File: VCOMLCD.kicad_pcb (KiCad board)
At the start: 2 copper layers, 123.2 x 44.5 mm, 49 parts, among them J1 Screw_Terminal_01x02, J2 USB_B_Mini, J3 Conn_01x05, J4 Conn_01x03, J5 Conn_01x06, Q1 BC847, SW1 SYS_RST, SW2 BTN, U1 MCP73831-2-OT, U2 MCP1700-3302E_SOT23, U3 74LVC4245A, U4 LCD-016N002L, U5 STM32F042F4Px, U6 ESP-12E

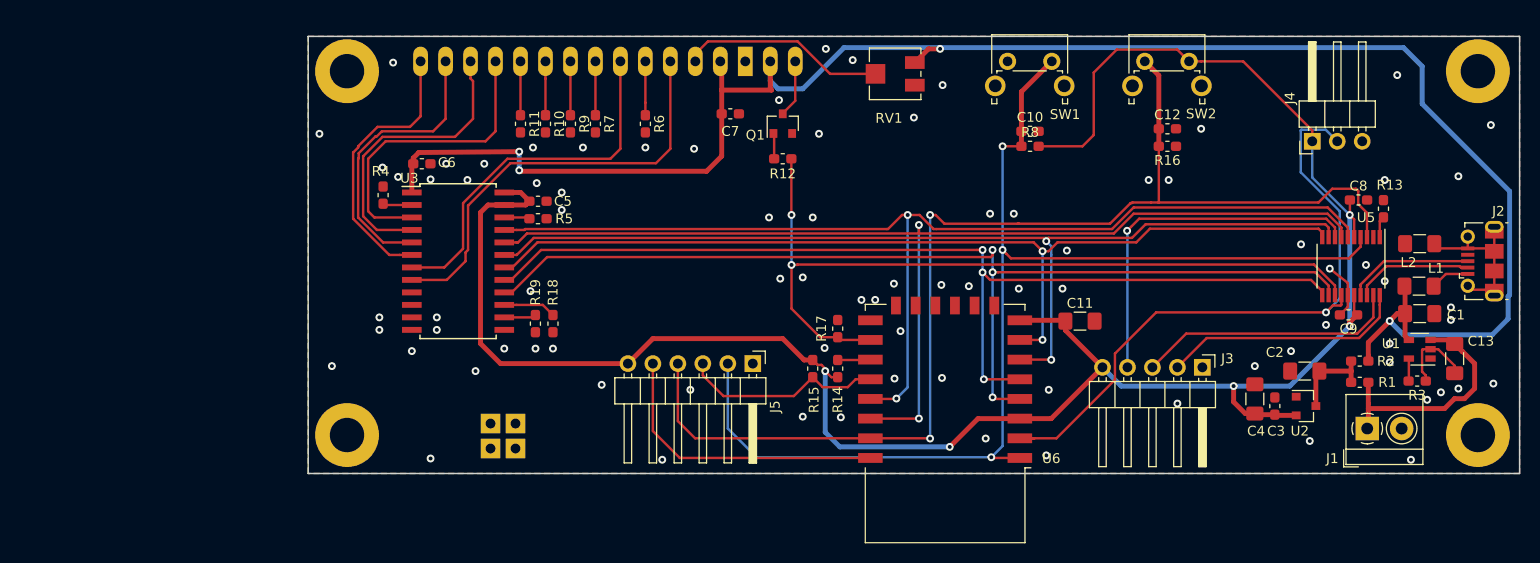
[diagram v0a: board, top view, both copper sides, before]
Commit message: pre-fabrication commit
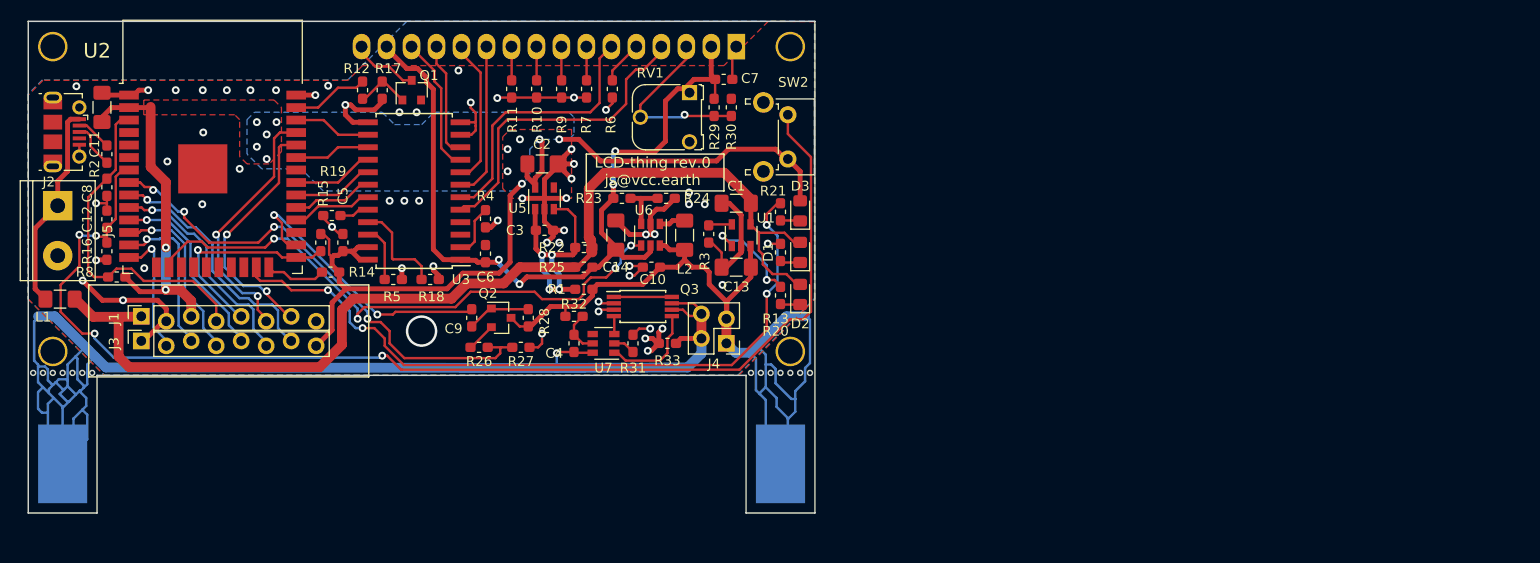
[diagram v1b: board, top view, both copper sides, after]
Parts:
- removed SW1: SYS_RST, Button_Switch_THT:SW_Tactile_SPST_Angled_PTS645Vx83-2LFS
- added C14: 10u, Capacitor_SMD:C_1206_3216Metric_Pad1.42x1.75mm_HandSolder, F.Cu at (108.8, 69.7)
- added D1: LED_RED, LED_SMD:LED_0805_2012Metric_Pad1.15x1.40mm_HandSolder, F.Cu at (127.5, 71.5)
- added D2: LED_GREEN, LED_SMD:LED_0805_2012Metric_Pad1.15x1.40mm_HandSolder, F.Cu at (127.5, 75.8)
- added D3: LED_BLUE, LED_SMD:LED_0805_2012Metric_Pad1.15x1.40mm_HandSolder, F.Cu at (127.5, 67.3)
- added Q2: AO3401A, Package_TO_SOT_SMD:SOT-23, F.Cu at (97.1, 78.2)
- added Q3: FS8205A, Package_SO:TSSOP-8_4.4x3mm_P0.65mm, F.Cu at (111.5, 77.0)
- added R20: 1k, Resistor_SMD:R_0603_1608Metric_Pad1.05x0.95mm_HandSolder, F.Cu at (125.5, 75.9)
- added R21: 200, Resistor_SMD:R_0603_1608Metric_Pad1.05x0.95mm_HandSolder, F.Cu at (125.5, 67.4)
- added R22: NC, Resistor_SMD:R_0603_1608Metric_Pad1.05x0.95mm_HandSolder, F.Cu at (105.5, 71.0)
- added R23: 698k, Resistor_SMD:R_0603_1608Metric_Pad1.05x0.95mm_HandSolder, F.Cu at (109.4, 66.0)
- added R24: 133k, Resistor_SMD:R_0603_1608Metric_Pad1.05x0.95mm_HandSolder, F.Cu at (113.9, 66.0)
- added R25: NC, Resistor_SMD:R_0603_1608Metric_Pad1.05x0.95mm_HandSolder, F.Cu at (105.5, 73.0)
- added R26: 10k/1%, Resistor_SMD:R_0603_1608Metric_Pad1.05x0.95mm_HandSolder, F.Cu at (94.8, 81.2)
- added R27: 10k/1%, Resistor_SMD:R_0603_1608Metric_Pad1.05x0.95mm_HandSolder, F.Cu at (99.1, 81.2)
- added R28: 10k, Resistor_SMD:R_0603_1608Metric_Pad1.05x0.95mm_HandSolder, F.Cu at (99.8, 78.2)
- added R29: NC, Resistor_SMD:R_0603_1608Metric_Pad1.05x0.95mm_HandSolder, F.Cu at (118.8, 56.8)
- added R30: NC, Resistor_SMD:R_0603_1608Metric_Pad1.05x0.95mm_HandSolder, F.Cu at (120.5, 56.8)
- added R31: 1k, Resistor_SMD:R_0603_1608Metric_Pad1.05x0.95mm_HandSolder, F.Cu at (110.5, 80.8)
- added R32: 200, Resistor_SMD:R_0603_1608Metric_Pad1.05x0.95mm_HandSolder, F.Cu at (104.5, 78.0)
- added R33: NC, Resistor_SMD:R_0603_1608Metric_Pad1.05x0.95mm_HandSolder, F.Cu at (114.0, 80.8)
- added TP1: Lipo+, TestPoint:TestPoint_Pad_1.0x1.0mm, B.Cu at (125.5, 93.0)
- added TP2: LiPo-, TestPoint:TestPoint_Pad_1.0x1.0mm, B.Cu at (52.5, 93.0)
- added U7: DW01x, Package_TO_SOT_SMD:SOT-23-6, F.Cu at (107.5, 80.8)
- C10, C3: value 100n -> 1u
- C11, C13, C2: value 22u -> 10u
- C4: value 22u -> 100n; footprint Capacitor_SMD:C_1206_3216Metric_Pad1.42x1.75mm_HandSolder -> Capacitor_SMD:C_0603_1608Metric_Pad1.05x0.95mm_HandSolder
- J1: value Screw_Terminal_01x02 -> Conn_01x08; footprint TerminalBlock_4Ucon:TerminalBlock_4Ucon_1x02_P3.50mm_Horizontal -> Connector_PinSocket_2.54mm:PinSocket_1x08_P2.54mm_Vertical
- J3: value Conn_01x05 -> Conn_01x08; footprint Connector_PinHeader_2.54mm:PinHeader_1x05_P2.54mm_Horizontal -> Connector_PinSocket_2.54mm:PinSocket_1x08_P2.54mm_Vertical
- J4: value Conn_01x03 -> LiPo_ext; footprint Connector_PinHeader_2.54mm:PinHeader_1x03_P2.54mm_Horizontal -> Connector_PinHeader_2.54mm:PinHeader_2x02_P2.54mm_Vertical
- J5: value Conn_01x06 -> Screw_Terminal_01x02; footprint Connector_PinHeader_2.54mm:PinHeader_1x06_P2.54mm_Horizontal -> TerminalBlock:TerminalBlock_bornier-2_P5.08mm
- L1: value L_Small -> 0R
- L2: value L_Small -> 10uH
- Q1: value BC847 -> BC817
- R1: value NC -> 0R
- R12, R16, R3, R8: value R -> 10k
- R13: value R -> 1k
- R2: value 0R -> 200
- RV1: footprint Potentiometer_SMD:Potentiometer_Vishay_TS53YJ_Vertical -> Potentiometer_THT:Potentiometer_Runtron_RM-065_Vertical
- U2: value MCP1700-3302E_SOT23 -> ESP32-WROOM-32; footprint Package_TO_SOT_SMD:SOT-23 -> RF_Module:ESP32-WROOM-32
- U4: footprint Display:LCD-016N002L -> Display:WC1602A
- U5: value STM32F042F4Px -> XC6220B331MR; footprint Package_SO:TSSOP-20_4.4x6.5mm_P0.65mm -> Package_TO_SOT_SMD:SOT-23-5
- U6: value ESP-12E -> TLV61046ADB; footprint RF_Module:ESP-12E -> Package_TO_SOT_SMD:SOT-23-6
- moved J2 144.7 mm to (52.7, 59.2), turned to 270 degrees
- moved L1 138.2 mm to (52.2, 76.2), turned to 180 degrees
- moved R2 129.1 mm to (57.0, 61.5), turned to 90 degrees
- moved C8 127.3 mm to (57.0, 64.9), turned to 270 degrees
- moved J1 125.2 mm to (60.5, 78.2), turned to 90 degrees
- moved U2 113.6 mm to (67.8, 63.8)
- moved R16 108.4 mm to (57.0, 71.4), turned to 90 degrees
- moved C12 108.2 mm to (57.0, 68.1), turned to 90 degrees
- moved J3 107.9 mm to (60.5, 80.8), turned to 90 degrees
- moved C11 101.8 mm to (56.5, 56.8), turned to 90 degrees
- moved R8 93.8 mm to (58.0, 74.0)
- moved C9 89.2 mm to (94.1, 78.2), turned to 90 degrees
- moved U5 82.3 mm to (101.5, 66.0), turned to 90 degrees
- moved C2 80.4 mm to (101.2, 62.5), turned to 0 degrees
- moved R1 79.5 mm to (105.5, 75.2)
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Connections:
- C10 pad 1: /ESP_RTS -> +BATT
- C2 pad 1: Net-(C2-Pad1) -> +3V3
- C3 pad 1: +3V3 -> Net-(C3-Pad1)
- C4 pad 1: +3V3 -> Net-(C4-Pad1)
- C4 pad 2: GND -> Net-(C4-Pad2)
- C6 pad 1: VBUS -> +5V
- C7 pad 1: VBUS -> +5V
- C8 pad 1: +3V3 -> /PROG_RTS
- C9 pad 1: +3V3 -> Net-(C9-Pad1)
- C9 pad 2: GND -> /LIPO_DIV_ENA
- J1 pad 1: +BATT -> VBUS
- J2 pad 5: Net-(J2-Pad5) -> GND
- J2 pad 6: Net-(J2-Pad5) -> GND
- J3 pad 2: /SWCLK -> /GPIO12
- J3 pad 3: /SWDIO -> /GPIO14
- J3 pad 4: /STM_TX -> /GPIO27
- J3 pad 5: +3V3 -> /GPIO26
- J4 pad 1: +3V3 -> +BATT
- J4 pad 2: Net-(J4-Pad2) -> Net-(C4-Pad2)
- J4 pad 3: GND -> +BATT
- J5 pad 1: GND -> Net-(J2-Pad1)
- J5 pad 2: /ESP_RTS -> GND
- L2 pad 1: Net-(J2-Pad5) -> +BATT
- L2 pad 2: GND -> Net-(L2-Pad2)
- R1 pad 1: Net-(C2-Pad1) -> Net-(C3-Pad1)
- R13 pad 1: GND -> Net-(D1-Pad1)
- R13 pad 2: Net-(R13-Pad2) -> GND
- R15 pad 1: /ESP_DTR -> /PROG_DTR
- R17 pad 2: /BL_CTRL -> Net-(Q1-Pad1)
- R2 pad 1: Net-(C2-Pad1) -> Net-(J2-Pad3)
- R2 pad 2: VBUS -> Net-(J2-Pad2)
- R8 pad 1: /ESP_RTS -> /PROG_RTS
- RV1 pad 1: VBUS -> +5V
- U2 pad 3: Net-(C2-Pad1) -> /PROG_RTS
- U3 pad 1: VBUS -> +5V
- U3 pad 14: Net-(R19-Pad2) -> /DB6_3V3
- U3 pad 15: Net-(R18-Pad2) -> /DB7_3V3
- U3 pad 16: Net-(U3-Pad16) -> /DB5_3V3
- U3 pad 17: Net-(U3-Pad17) -> /DB4_3V3
- U3 pad 18: Net-(U3-Pad18) -> /E_3V3
- U3 pad 19: Net-(U3-Pad19) -> /RS_3V3
- U3 pad 20: Net-(U3-Pad20) -> Net-(R19-Pad2)
- U3 pad 21: Net-(U3-Pad21) -> Net-(R18-Pad2)
- U4 pad 11: Net-(U3-Pad3) -> Net-(U3-Pad7)
- U4 pad 12: Net-(U3-Pad4) -> Net-(U3-Pad8)
- U4 pad 13: Net-(U3-Pad5) -> Net-(U3-Pad10)
- U4 pad 14: Net-(U3-Pad6) -> Net-(U3-Pad9)
- U4 pad 15: VBUS -> +5V
- U4 pad 2: VBUS -> +5V
- U4 pad 4: Net-(U3-Pad8) -> Net-(U3-Pad5)
- U4 pad 6: Net-(U3-Pad7) -> Net-(U3-Pad6)
- U5 pad 1: Net-(R13-Pad2) -> Net-(C3-Pad1)
- U5 pad 2: Net-(U5-Pad2) -> GND
- U5 pad 3: /BTN -> Net-(C3-Pad1)
- U5 pad 4: /ESP_RTS -> Net-(U5-Pad4)
- U6 pad 1: /ESP_RTS -> Net-(L2-Pad2)
- U6 pad 2: Net-(J4-Pad2) -> GND
- U6 pad 3: +3V3 -> Net-(R23-Pad2)
- U6 pad 4: Net-(U3-Pad16) -> /5V_ENA
- U6 pad 5: Net-(U3-Pad17) -> +5V
- U6 pad 6: Net-(U3-Pad19) -> +BATT
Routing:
- net Net-(C4-Pad2): track 0.00 -> 158.6 mm, vias 0 -> 1
- net /ESP_RTS: track 119.7 -> 0.00 mm, vias 3 -> 0
- net Net-(U3-Pad20): track 113.4 -> 0.00 mm, vias 2 -> 0
- net Net-(U3-Pad21): track 111.5 -> 0.00 mm, vias 2 -> 0
- net GND: track 14.0 -> 121.2 mm, vias 84 -> 57
- net Net-(U3-Pad16): track 105.3 -> 0.00 mm, vias 3 -> 0
- net Net-(U3-Pad17): track 102.5 -> 0.00 mm, vias 3 -> 0
- net Net-(U3-Pad19): track 102.2 -> 0.00 mm, vias 2 -> 0
- net +3V3: track 216.9 -> 118.9 mm, vias 5 -> 13
- net Net-(U3-Pad18): track 97.5 -> 0.00 mm, vias 2 -> 0
- net +5V: track 0.00 -> 82.3 mm, vias 0 -> 4
- net +BATT: track 24.4 -> 101.2 mm
- net VBUS: track 185.2 -> 108.7 mm, vias 4 -> 0
- net /BL_CTRL: track 81.7 -> 7.85 mm, vias 2 -> 0
- net Net-(R21-Pad1): track 0.00 -> 73.8 mm, vias 0 -> 4
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- added copper zone on B.Cu, net +3V3
- added copper zone on F.Cu, net +3V3
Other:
- board size 123.2 x 44.5 mm -> 80 x 50 mm
- board text added: "LCD-thing rev.0 js@vcc.earth"
